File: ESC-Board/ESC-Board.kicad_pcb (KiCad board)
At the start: 2 copper layers, 17.1 x 32 mm, 26 parts, among them J1 Molex, J2 Molex, J3 XT_60, U1 ESC:Blue_ESC, U2 ESC:Blue_ESC, U3 ESC:Blue_ESC, U4 ESC:Blue_ESC

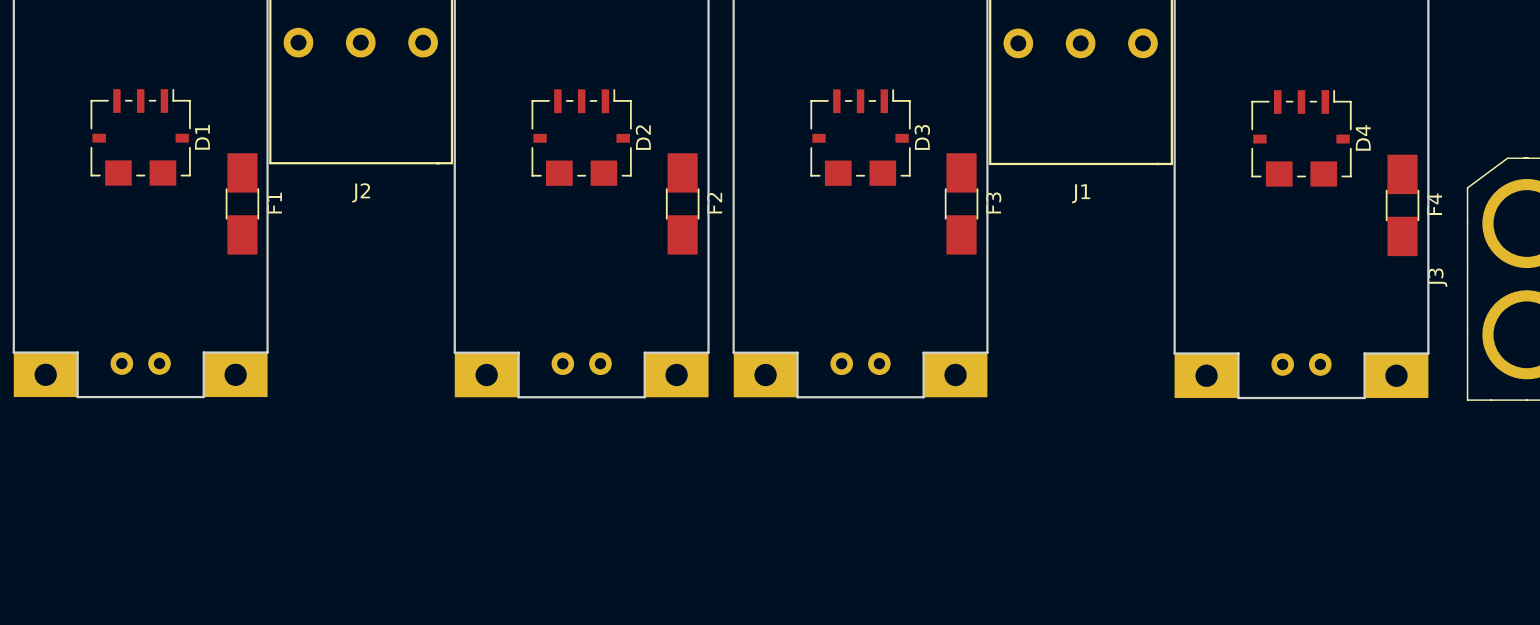
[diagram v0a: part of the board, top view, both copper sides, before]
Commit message: Cur
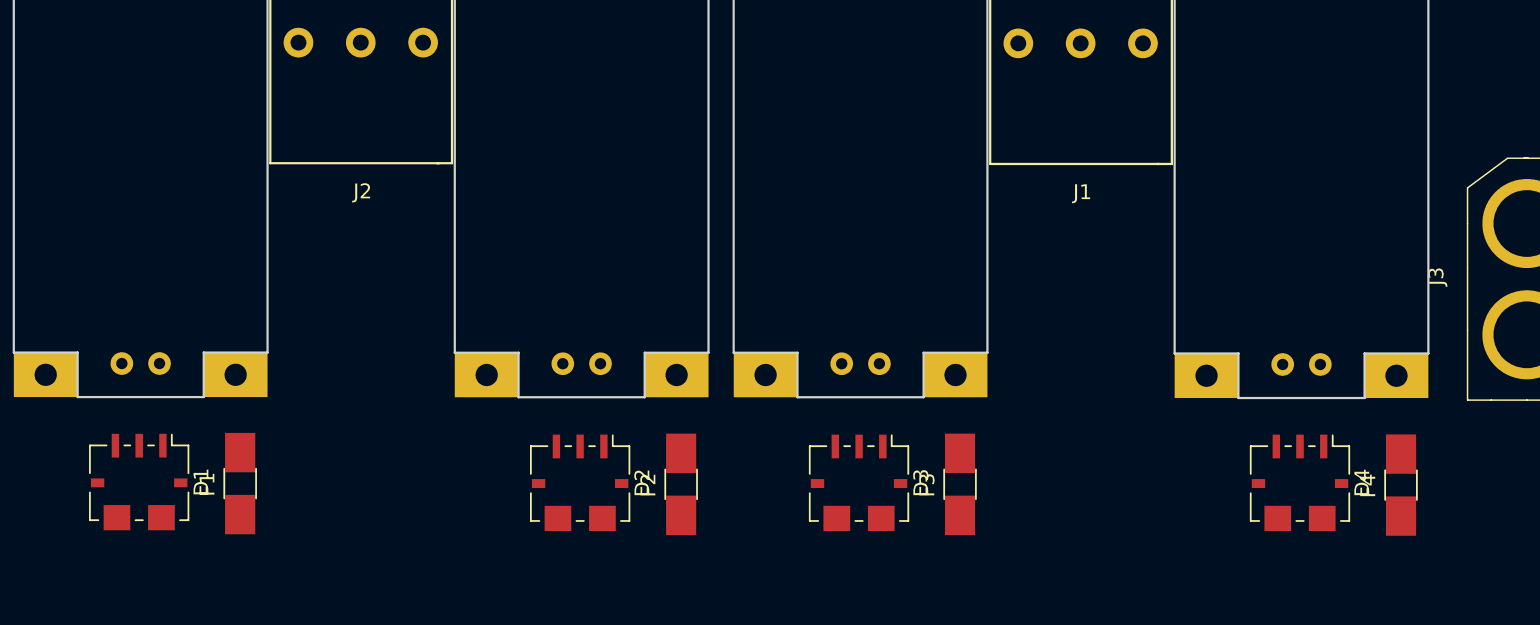
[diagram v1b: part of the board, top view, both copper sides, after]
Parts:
- moved D2 23.3 mm to (76.9, 103.0)
- moved D3 23.3 mm to (95.7, 103.0)
- moved D1 23.2 mm to (47.1, 102.9)
- moved D4 23.2 mm to (125.4, 103.0)
- moved F2 18.9 mm to (83.7, 103.1), turned to 90 degrees
- moved F3 18.9 mm to (102.5, 103.1), turned to 90 degrees
- moved F1 18.8 mm to (53.9, 103.0), turned to 90 degrees
- moved F4 18.8 mm to (132.2, 103.1), turned to 90 degrees
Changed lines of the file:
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@@
   )
   (module Blue_ESC:Allegro_PSOF-7_4.8x6.4mm_Pitch1.60mm (layer F.Cu)
-    (at 47.244 79.6925 270)
+    (at 47.1424 102.9208 270)
     (descr "Allegro Microsystems PSOF-7, 4.8x6.4mm Body, 1.60mm Pitch (http://www.allegromicro.com/~/media/Files/Datasheets/ACS780-Datasheet.ashx)")
     (tags "Allegro PSOF-7")
@@
     (fp_line (start -0.6 3.32) (end -2.47 3.32) (layer F.SilkS) (width 0.12))
     (fp_line (start 2.57 3.32) (end 0.7 3.32) (layer F.SilkS) (width 0.12))
-    (fp_text user %R (at 0 0 270) (layer F.Fab)
+    (fp_text user %R (at 0 0) (layer F.Fab)
       (effects (font (size 1 1) (thickness 0.15)))
     )
@@
   )
   (module Blue_ESC:Allegro_PSOF-7_4.8x6.4mm_Pitch1.60mm (layer F.Cu)
-    (at 76.962 79.7052 270)
+    (at 76.8604 102.9716 270)
     (descr "Allegro Microsystems PSOF-7, 4.8x6.4mm Body, 1.60mm Pitch (http://www.allegromicro.com/~/media/Files/Datasheets/ACS780-Datasheet.ashx)")
     (tags "Allegro PSOF-7")
@@
   )
   (module Blue_ESC:Allegro_PSOF-7_4.8x6.4mm_Pitch1.60mm (layer F.Cu)
-    (at 95.758 79.7052 270)
+    (at 95.6564 102.9716 270)
     (descr "Allegro Microsystems PSOF-7, 4.8x6.4mm Body, 1.60mm Pitch (http://www.allegromicro.com/~/media/Files/Datasheets/ACS780-Datasheet.ashx)")
     (tags "Allegro PSOF-7")
@@
   )
   (module Blue_ESC:Allegro_PSOF-7_4.8x6.4mm_Pitch1.60mm (layer F.Cu)
-    (at 125.476 79.756 270)
+    (at 125.3744 102.9716 270)
     (descr "Allegro Microsystems PSOF-7, 4.8x6.4mm Body, 1.60mm Pitch (http://www.allegromicro.com/~/media/Files/Datasheets/ACS780-Datasheet.ashx)")
     (tags "Allegro PSOF-7")
@@
   )
   (module Fuse_Holders_and_Fuses:Fuse_SMD1206_HandSoldering (layer F.Cu)
-    (at 54.102 84.1756 270)
+    (at 53.9496 103.0224 90)
     (descr "Fuse, Sicherung, SMD1206, Littlefuse-Wickmann 433 Series, Hand Soldering,")
     (tags "Fuse Sicherung SMD1206 Littlefuse-Wickmann 433 Series Hand Soldering ")
     (attr smd)
-    (fp_text reference F1 (at -0.05 -2.2 270) (layer F.SilkS)
-      (effects (font (size 1 1) (thickness 0.15)))
-    )
-    (fp_text value 10/15 (at -0.15 2.5 270) (layer F.Fab)
+    (fp_text reference F1 (at -0.05 -2.2 90) (layer F.SilkS)
+      (effects (font (size 1 1) (thickness 0.15)))
+    )
+    (fp_text value 10/15 (at -0.15 2.5 90) (layer F.Fab)
       (effects (font (size 1 1) (thickness 0.15)))
     )
@@
     (fp_line (start 3.35 1.58) (end 3.35 -1.58) (layer F.CrtYd) (width 0.05))
     (fp_line (start 3.35 1.58) (end -3.35 1.58) (layer F.CrtYd) (width 0.05))
-    (pad 1 smd rect (at -2.09 0) (size 2.03 2.65) (layers F.Cu F.Paste F.Mask)
+    (pad 1 smd rect (at -2.09 0 180) (size 2.03 2.65) (layers F.Cu F.Paste F.Mask)
       (net 1 "Net-(D1-Pad6)"))
-    (pad 2 smd rect (at 2.09 0) (size 2.03 2.65) (layers F.Cu F.Paste F.Mask)
+    (pad 2 smd rect (at 2.09 0 180) (size 2.03 2.65) (layers F.Cu F.Paste F.Mask)
       (net 23 +12V))
   )
   (module Fuse_Holders_and_Fuses:Fuse_SMD1206_HandSoldering (layer F.Cu)
-    (at 83.7692 84.1756 270)
+    (at 83.6676 103.0732 90)
     (descr "Fuse, Sicherung, SMD1206, Littlefuse-Wickmann 433 Series, Hand Soldering,")
     (tags "Fuse Sicherung SMD1206 Littlefuse-Wickmann 433 Series Hand Soldering ")
     (attr smd)
-    (fp_text reference F2 (at -0.05 -2.2 270) (layer F.SilkS)
-      (effects (font (size 1 1) (thickness 0.15)))
-    )
-    (fp_text value 10/15 (at -0.15 2.5 270) (layer F.Fab)
+    (fp_text reference F2 (at -0.05 -2.2 90) (layer F.SilkS)
+      (effects (font (size 1 1) (thickness 0.15)))
+    )
+    (fp_text value 10/15 (at -0.15 2.5 90) (layer F.Fab)
       (effects (font (size 1 1) (thickness 0.15)))
     )
@@
     (fp_line (start 1.6 0.8) (end -1.6 0.8) (layer F.Fab) (width 0.1))
     (fp_line (start -1.6 0.8) (end -1.6 -0.8) (layer F.Fab) (width 0.1))
-    (pad 2 smd rect (at 2.09 0) (size 2.03 2.65) (layers F.Cu F.Paste F.Mask)
+    (pad 2 smd rect (at 2.09 0 180) (size 2.03 2.65) (layers F.Cu F.Paste F.Mask)
       (net 23 +12V))
-    (pad 1 smd rect (at -2.09 0) (size 2.03 2.65) (layers F.Cu F.Paste F.Mask)
+    (pad 1 smd rect (at -2.09 0 180) (size 2.03 2.65) (layers F.Cu F.Paste F.Mask)
       (net 12 "Net-(D2-Pad6)"))
   )
   (module Fuse_Holders_and_Fuses:Fuse_SMD1206_HandSoldering (layer F.Cu)
-    (at 102.5652 84.1756 270)
+    (at 102.4636 103.0732 90)
     (descr "Fuse, Sicherung, SMD1206, Littlefuse-Wickmann 433 Series, Hand Soldering,")
     (tags "Fuse Sicherung SMD1206 Littlefuse-Wickmann 433 Series Hand Soldering ")
     (attr smd)
-    (fp_text reference F3 (at -0.05 -2.2 270) (layer F.SilkS)
-      (effects (font (size 1 1) (thickness 0.15)))
-    )
-    (fp_text value 10/15 (at -0.15 2.5 270) (layer F.Fab)
+    (fp_text reference F3 (at -0.05 -2.2 90) (layer F.SilkS)
+      (effects (font (size 1 1) (thickness 0.15)))
+    )
+    (fp_text value 10/15 (at -0.15 2.5 90) (layer F.Fab)
       (effects (font (size 1 1) (thickness 0.15)))
     )
@@
     (fp_line (start 3.35 1.58) (end 3.35 -1.58) (layer F.CrtYd) (width 0.05))
     (fp_line (start 3.35 1.58) (end -3.35 1.58) (layer F.CrtYd) (width 0.05))
-    (pad 1 smd rect (at -2.09 0) (size 2.03 2.65) (layers F.Cu F.Paste F.Mask)
+    (pad 1 smd rect (at -2.09 0 180) (size 2.03 2.65) (layers F.Cu F.Paste F.Mask)
       (net 13 "Net-(D3-Pad6)"))
-    (pad 2 smd rect (at 2.09 0) (size 2.03 2.65) (layers F.Cu F.Paste F.Mask)
+    (pad 2 smd rect (at 2.09 0 180) (size 2.03 2.65) (layers F.Cu F.Paste F.Mask)
       (net 23 +12V))
   )
   (module Fuse_Holders_and_Fuses:Fuse_SMD1206_HandSoldering (layer F.Cu)
-    (at 132.2832 84.2772 270)
+    (at 132.1816 103.124 90)
     (descr "Fuse, Sicherung, SMD1206, Littlefuse-Wickmann 433 Series, Hand Soldering,")
     (tags "Fuse Sicherung SMD1206 Littlefuse-Wickmann 433 Series Hand Soldering ")
     (attr smd)
-    (fp_text reference F4 (at -0.05 -2.2 270) (layer F.SilkS)
-      (effects (font (size 1 1) (thickness 0.15)))
-    )
-    (fp_text value 10/15 (at -0.15 2.5 270) (layer F.Fab)
+    (fp_text reference F4 (at -0.05 -2.2 90) (layer F.SilkS)
+      (effects (font (size 1 1) (thickness 0.15)))
+    )
+    (fp_text value 10/15 (at -0.15 2.5 90) (layer F.Fab)
       (effects (font (size 1 1) (thickness 0.15)))
     )
@@
     (fp_line (start 1.6 0.8) (end -1.6 0.8) (layer F.Fab) (width 0.1))
     (fp_line (start -1.6 0.8) (end -1.6 -0.8) (layer F.Fab) (width 0.1))
-    (pad 2 smd rect (at 2.09 0) (size 2.03 2.65) (layers F.Cu F.Paste F.Mask)
+    (pad 2 smd rect (at 2.09 0 180) (size 2.03 2.65) (layers F.Cu F.Paste F.Mask)
       (net 23 +12V))
-    (pad 1 smd rect (at -2.09 0) (size 2.03 2.65) (layers F.Cu F.Paste F.Mask)
+    (pad 1 smd rect (at -2.09 0 180) (size 2.03 2.65) (layers F.Cu F.Paste F.Mask)
       (net 22 "Net-(D4-Pad6)"))
   )

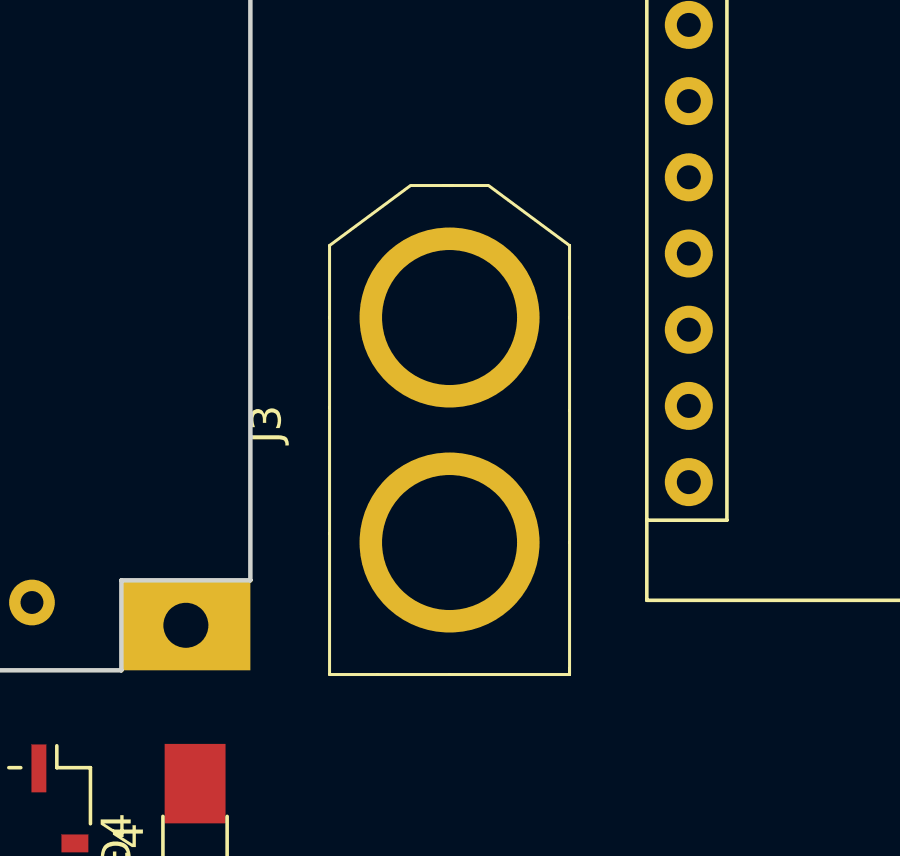
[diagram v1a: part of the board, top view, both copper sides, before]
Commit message: e
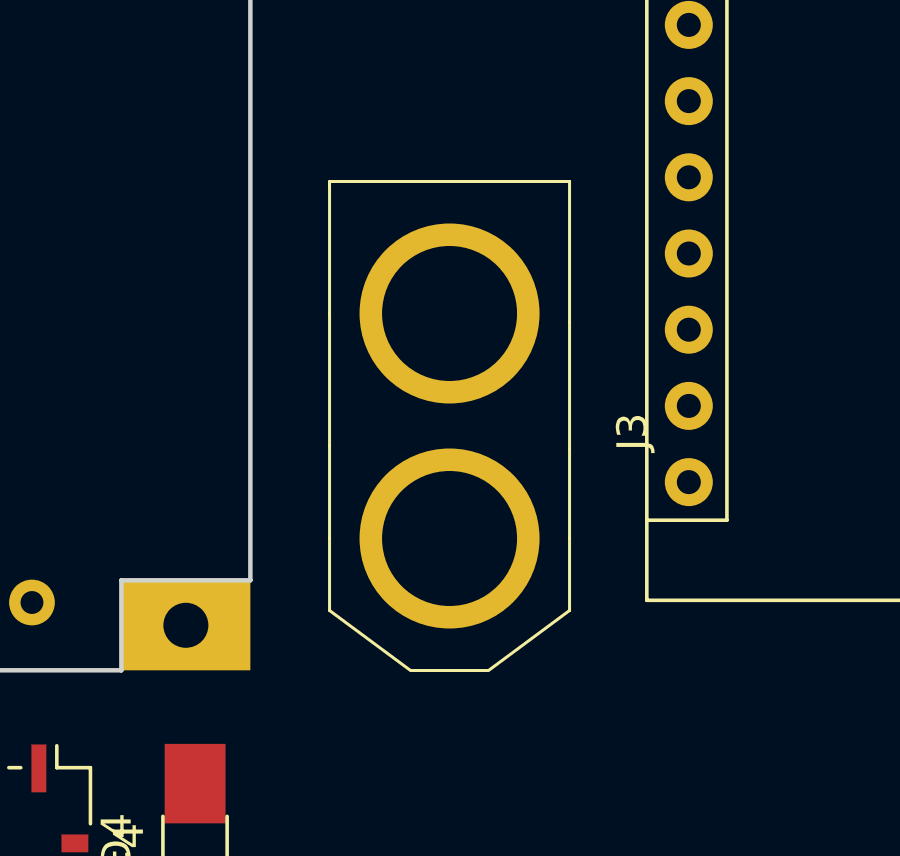
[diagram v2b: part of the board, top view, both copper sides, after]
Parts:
- moved J3 7.37 mm to (140.7, 92.9), turned to 90 degrees
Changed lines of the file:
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@@
   )
   (module Blue_ESC:XT60 (layer F.Cu)
-    (at 140.6652 85.4964 270)
-    (fp_text reference J3 (at 3.556 6.096 270) (layer F.SilkS)
+    (at 140.6652 92.8624 90)
+    (fp_text reference J3 (at 3.556 6.096 90) (layer F.SilkS)
       (effects (font (size 1 1) (thickness 0.15)))
     )
-    (fp_text value XT_60 (at 3.2 -5.9 270) (layer F.Fab)
+    (fp_text value XT_60 (at 3.2 -5.9 90) (layer F.Fab)
       (effects (font (size 1 1) (thickness 0.15)))
     )
@@
     (fp_line (start 7.5 -4) (end 3.1 -4) (layer F.SilkS) (width 0.1))
     (fp_line (start 7.2 4) (end 3 4) (layer F.SilkS) (width 0.1))
-    (pad 1 thru_hole circle (at 0 0 270) (size 6 6) (drill 4.5) (layers *.Cu *.Mask F.SilkS)
+    (pad 1 thru_hole circle (at 0 0 90) (size 6 6) (drill 4.5) (layers *.Cu *.Mask F.SilkS)
       (net 23 +12V))
-    (pad 2 thru_hole circle (at 7.5 0 270) (size 6 6) (drill 4.5) (layers *.Cu *.Mask F.SilkS)
+    (pad 2 thru_hole circle (at 7.5 0 90) (size 6 6) (drill 4.5) (layers *.Cu *.Mask F.SilkS)
       (net 6 GND))
   )

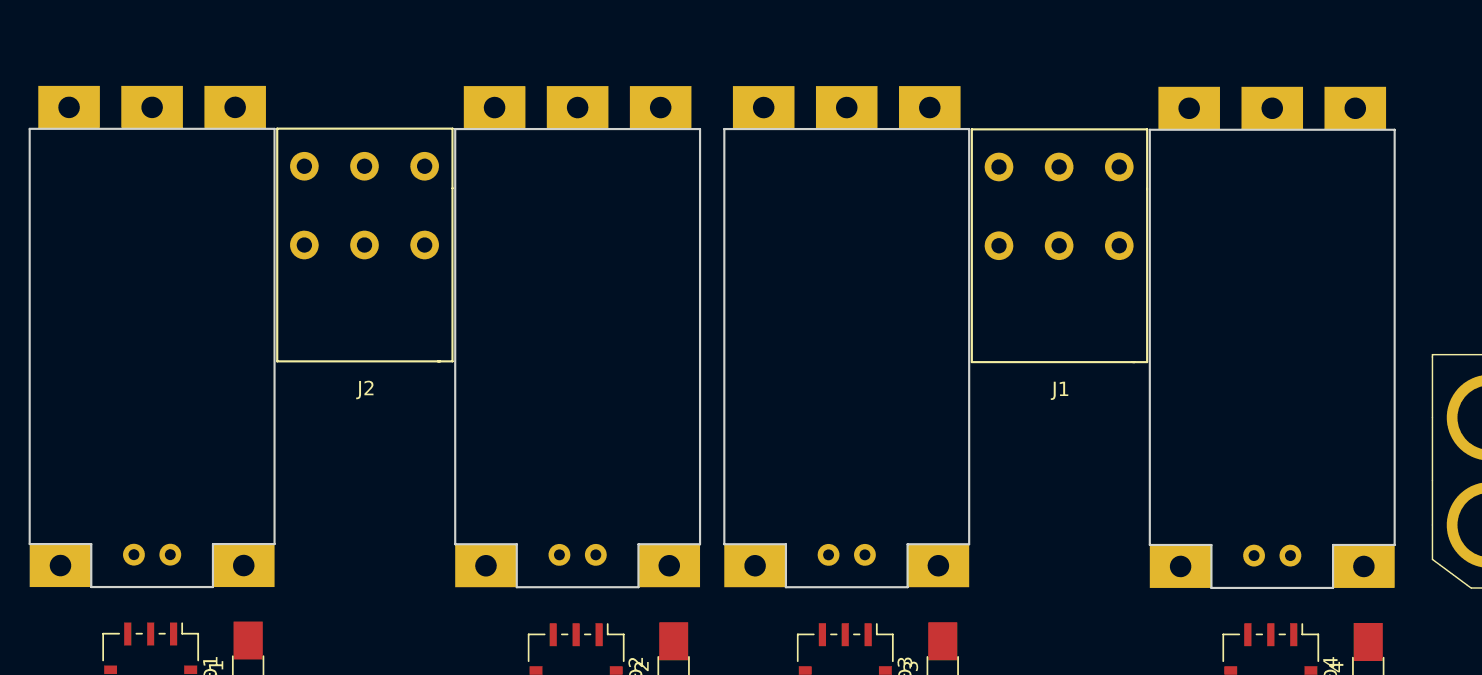
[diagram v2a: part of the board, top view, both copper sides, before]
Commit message: w
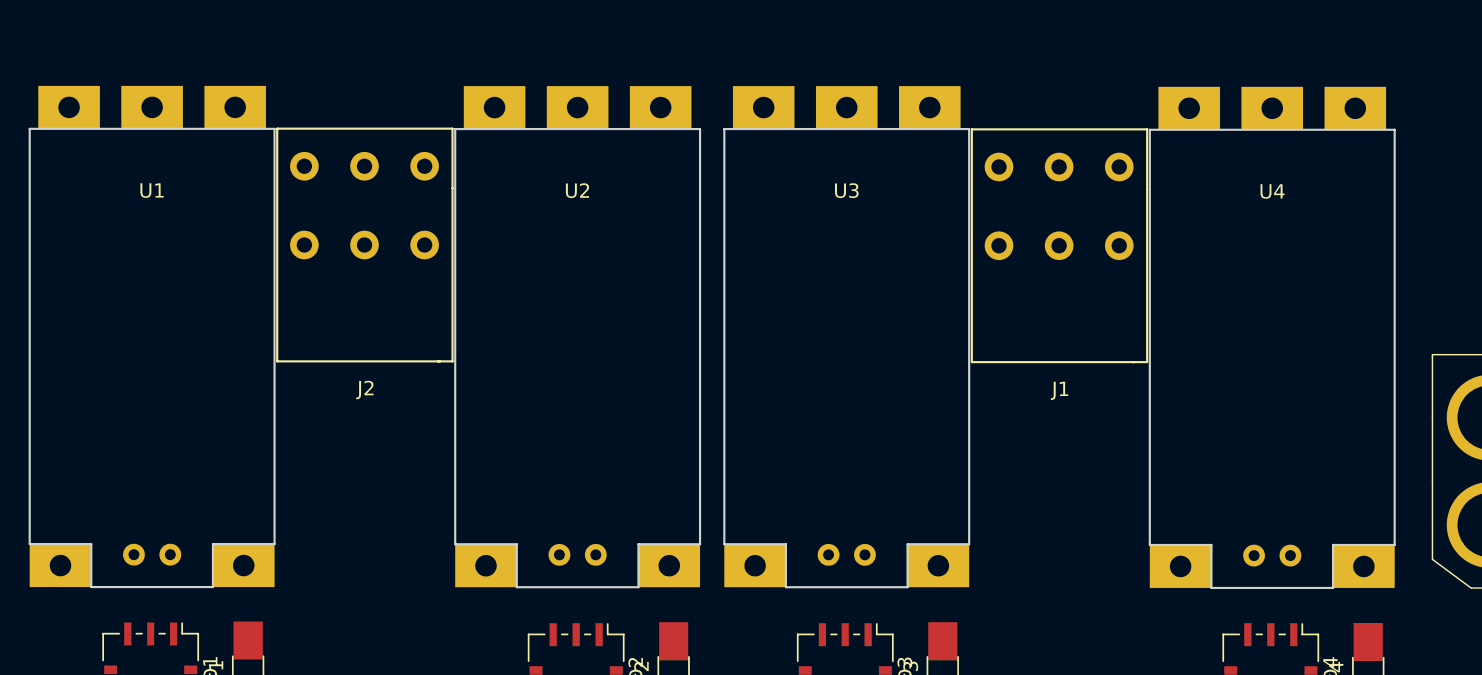
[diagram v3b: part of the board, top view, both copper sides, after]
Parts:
- U1, U2, U3, U4: moved to F.Cu
- turned U1 to 180 degrees
- turned U2 to 180 degrees
- turned U3 to 180 degrees
- turned U4 to 180 degrees
